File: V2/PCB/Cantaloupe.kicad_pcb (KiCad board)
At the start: 2 copper layers, 143.9 x 118.7 mm, 121 parts, among them J1 USB_In, J2 OLED, J3 Link, J4 Debug, J5 Trackball, Q1 2N7002, Q2 AO3401A, SW1 MX, SW10 MX, SW11 MX, SW12 MX, SW13 MX, SW14 MX, SW15 MX, SW16 MX, SW17 MX, SW18 MX, SW19 MX, SW2 MX, SW20 MX, SW21 MX, SW22 MX, SW23 MX, SW24 MX, SW25 MX, SW26 MX, SW27 MX, SW28 MX, SW29 MX, SW3 MX, SW30 MX, SW31 Encoder, SW32 MX, SW4 MX, SW5 MX, SW6 MX, SW7 MX, SW8 MX, SW9 MX, U1 STM32F4x1CxUx, U2 SRV0504, U3 SRV0504, U4 XC6206P332MR, U5 LMV321, Y1 8MHz

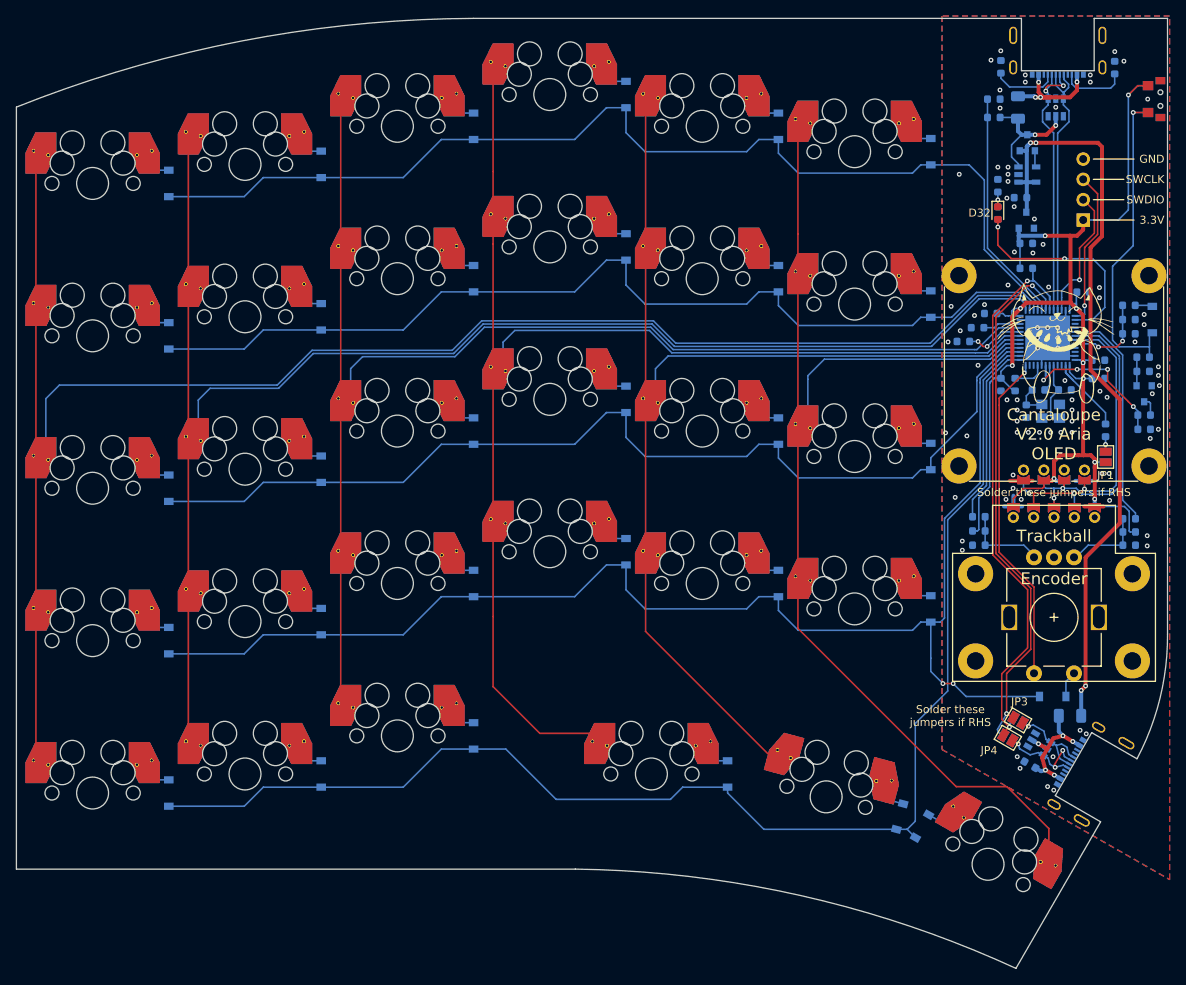
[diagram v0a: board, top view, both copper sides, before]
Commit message: Tentative V2.1 update
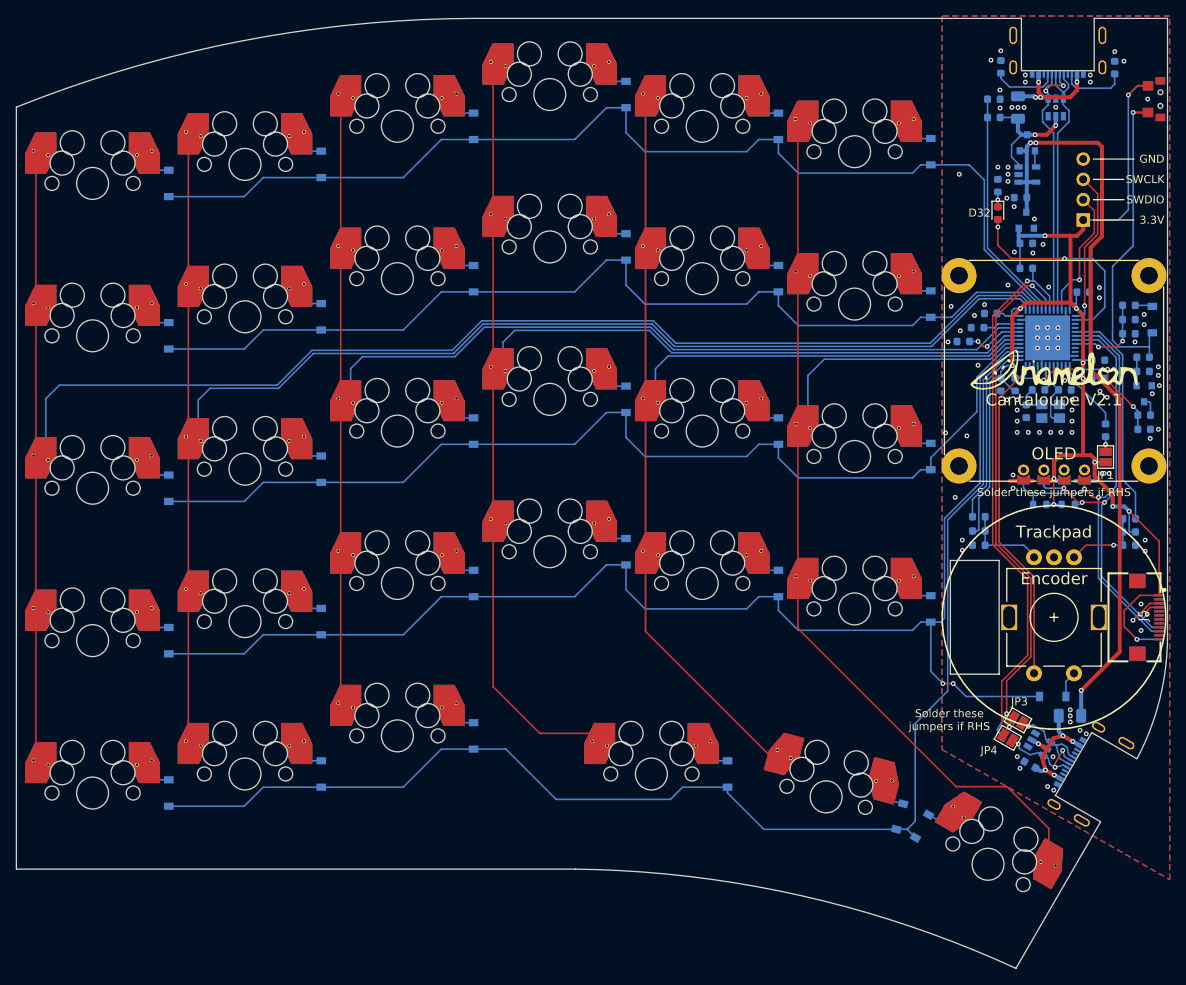
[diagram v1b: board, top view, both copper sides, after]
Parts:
- added R19: 4.7k, Resistor_SMD:R_0603_1608Metric, B.Cu at (144.8, 74.4)
- added R20: 4.7k, Resistor_SMD:R_0603_1608Metric, B.Cu at (141.3, 74.4)
- A1: footprint Ariamelon:Catmelon -> Ariamelon:Ariamelon_Logo_x2
- J5: value Trackball -> Trackpad; footprint Ariamelon:pimoroni_trackball_flippable -> Ariamelon:FPC-SMD_FPC05012-09200-.5mm-rev
- moved J5 11.8 mm to (154.8, 88.5)
- moved A1 5.58 mm to (143.0, 57.5)
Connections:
- J5 pad 2: SDA -> GND
- J5 pad 3: SCL -> SDA
- J5 pad 5: GND -> unconnected-(J5-Pad5)
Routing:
- net SDA: track 39.6 -> 63.7 mm
- net VDD: track 162.4 -> 182.4 mm, vias 10 -> 13
- net SCL: track 38.9 -> 58.8 mm, vias 2 -> 4
- net GND: track 30.0 -> 13.2 mm, vias 88 -> 93
- net Side: track 11.7 -> 9.40 mm
- net Net-(D24-Pad2): track 2.81 -> 1.55 mm
- net Net-(D20-Pad2): track 2.81 -> 1.55 mm
- net Net-(D12-Pad2): track 2.81 -> 1.55 mm
- net Net-(D3-Pad2): track 2.81 -> 1.55 mm
- net Net-(D21-Pad2): track 2.81 -> 1.55 mm
- net Net-(D2-Pad2): track 2.81 -> 1.55 mm
- net Net-(D18-Pad2): track 2.81 -> 1.55 mm
- net Net-(D13-Pad2): track 2.81 -> 1.55 mm
- net Net-(D1-Pad2): track 2.81 -> 1.55 mm
- net Net-(D6-Pad2): track 2.81 -> 1.55 mm
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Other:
- outline, holes or cut-outs redrawn
- board text added: "Cantaloupe V2.1"
- board text added: "Trackpad"
- board text removed: "Cantaloupe V2.0 Aria"
- board text removed: "Trackball"
